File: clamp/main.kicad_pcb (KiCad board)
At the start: 2 copper layers, 80 parts, among them P1 CONN_01X12, P2 CONN_01X15, P3 CONN_01X03, P4 CONN_01X08, Q1 2N3904, U1 LM741, U12 LTZ1000, U13 LM741, U14 LM741, U2 LM741, U3 LM741, U4 LM741, U5 LM741, U6 LM741, U7 LM741

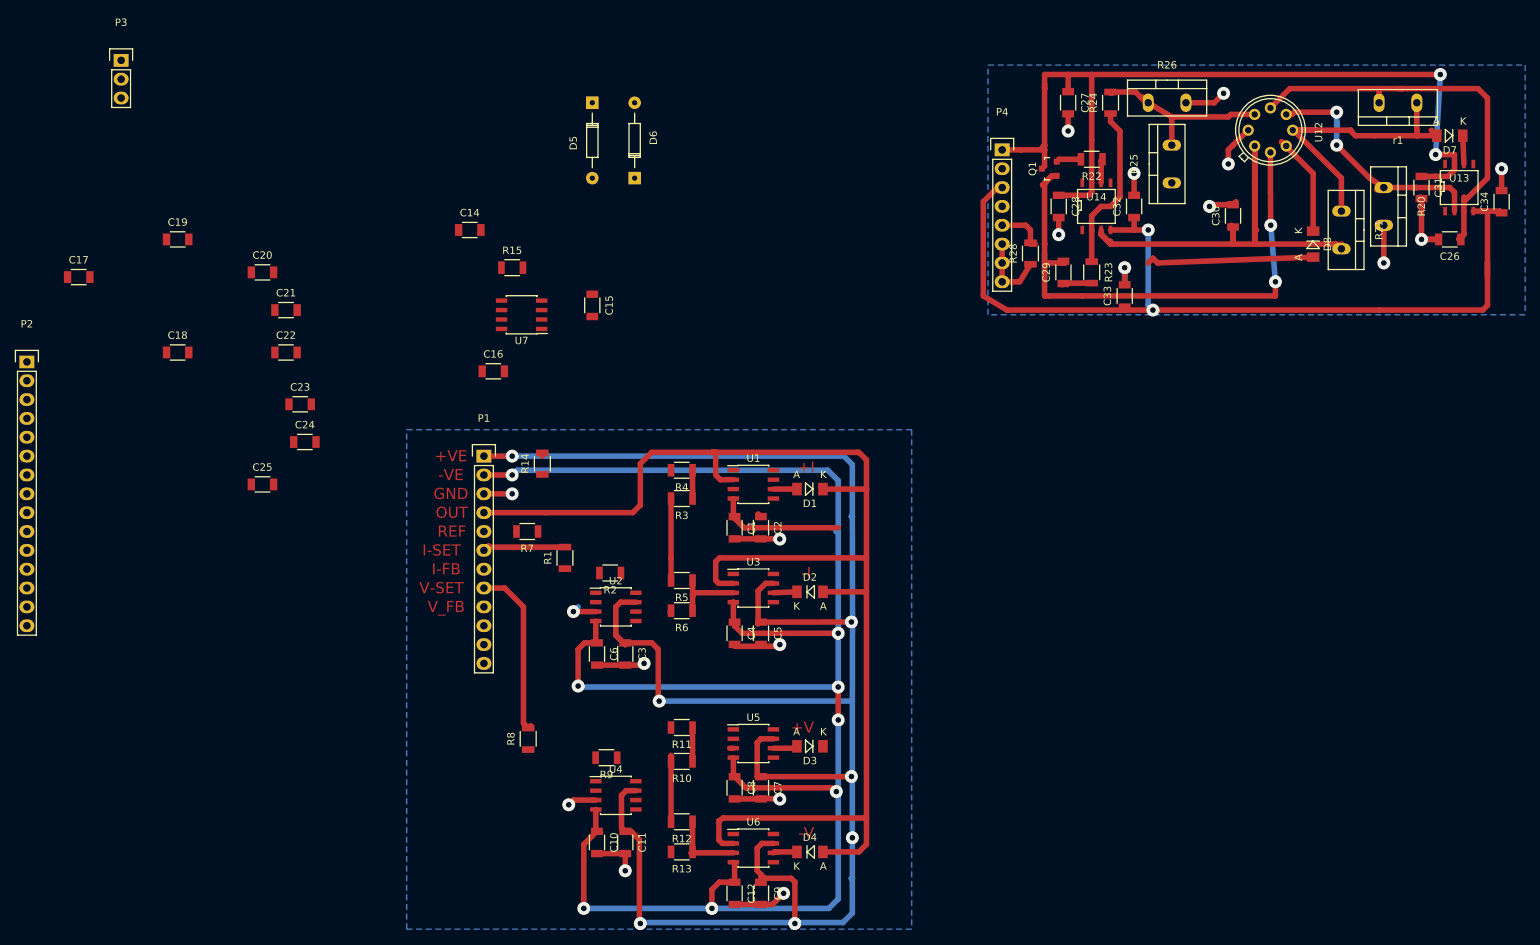
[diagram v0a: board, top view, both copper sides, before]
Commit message: update
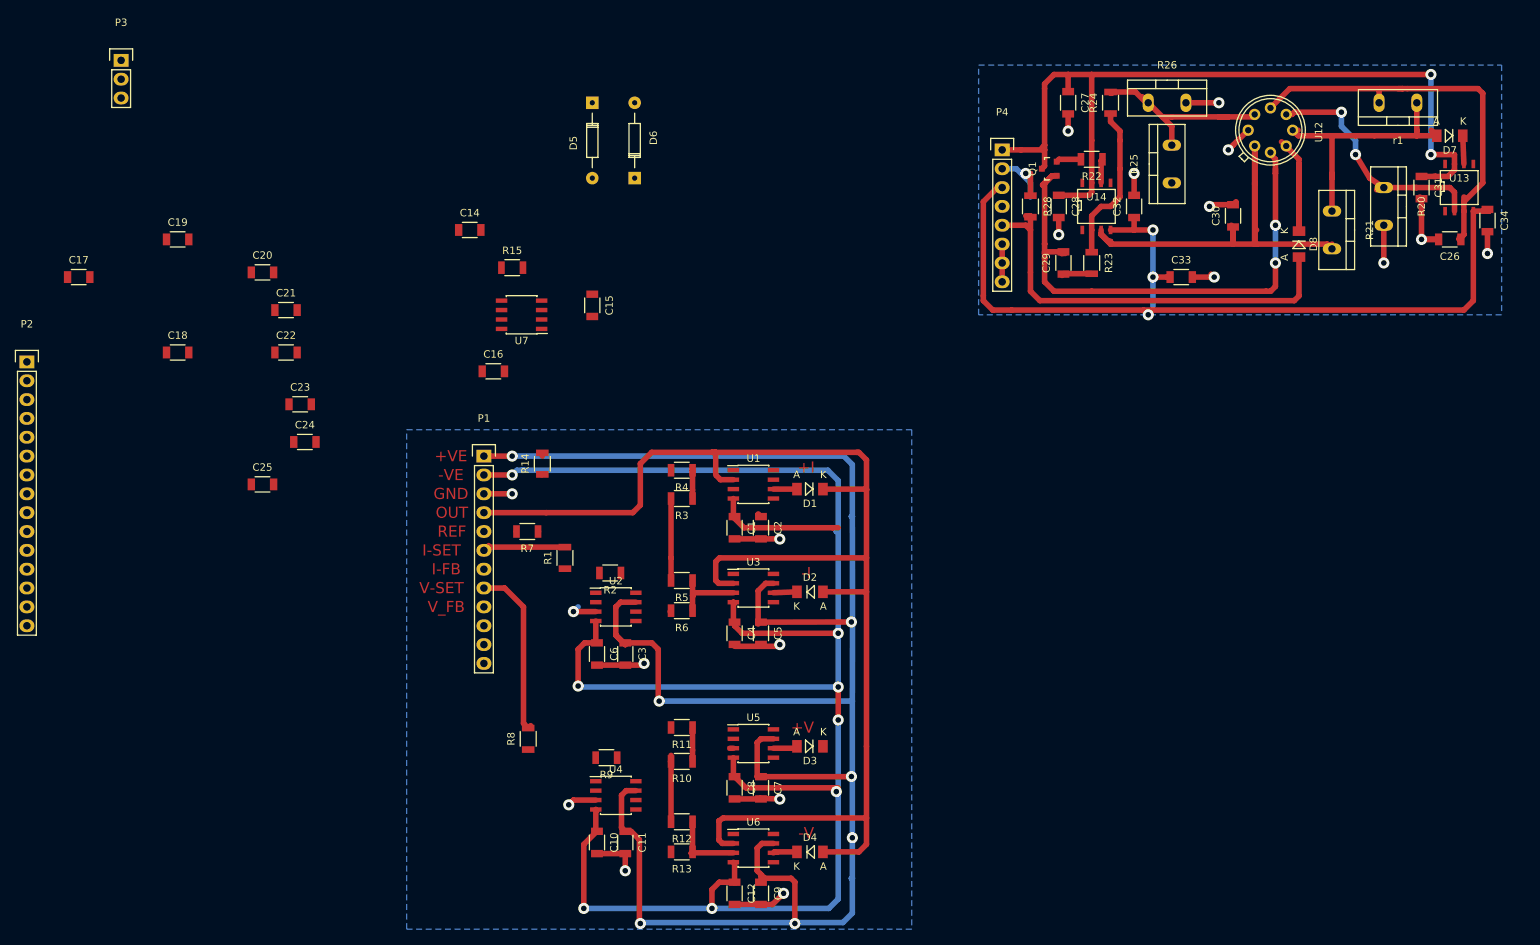
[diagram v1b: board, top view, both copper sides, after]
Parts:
- moved C33 8.03 mm to (212.1, 62.2), turned to 0 degrees
- moved R28 6.35 mm to (191.8, 52.7), turned to 270 degrees
- moved C34 3.18 mm to (253.4, 54.6), turned to 270 degrees
- moved D8 1.91 mm to (228.0, 57.8)
- moved R21 1.27 mm to (232.4, 55.9)
- moved C29 1.27 mm to (196.2, 60.3)
- moved R23 1.27 mm to (200.0, 60.3)
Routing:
- net GND-H: track 29.5 -> 57.2 mm
- net Net-(D8-Pad1): track 14.9 -> 22.2 mm
- net REF: track 43.7 -> 37.5 mm
- net (no net): track 3.40 -> 0.23 mm
- net Net-(R24-Pad2): track 27.2 -> 29.3 mm
- net +VE: track 399.6 -> 397.5 mm
- net Net-(C29-Pad2): track 73.7 -> 72.2 mm
- net Net-(R23-Pad1): track 23.3 -> 22.0 mm
- net Net-(C30-Pad1): track 69.8 -> 68.5 mm
- net GND: track 101.0 -> 101.7 mm, vias 18 -> 19
- net Net-(C26-Pad1): track 55.2 -> 54.7 mm
- net Net-(R20-Pad1): track 34.6 -> 34.0 mm
- net -VE: track 373.9 -> 373.4 mm, vias 10 -> 11
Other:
- net class Default: via_dia 1.75 -> 1.5

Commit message: update
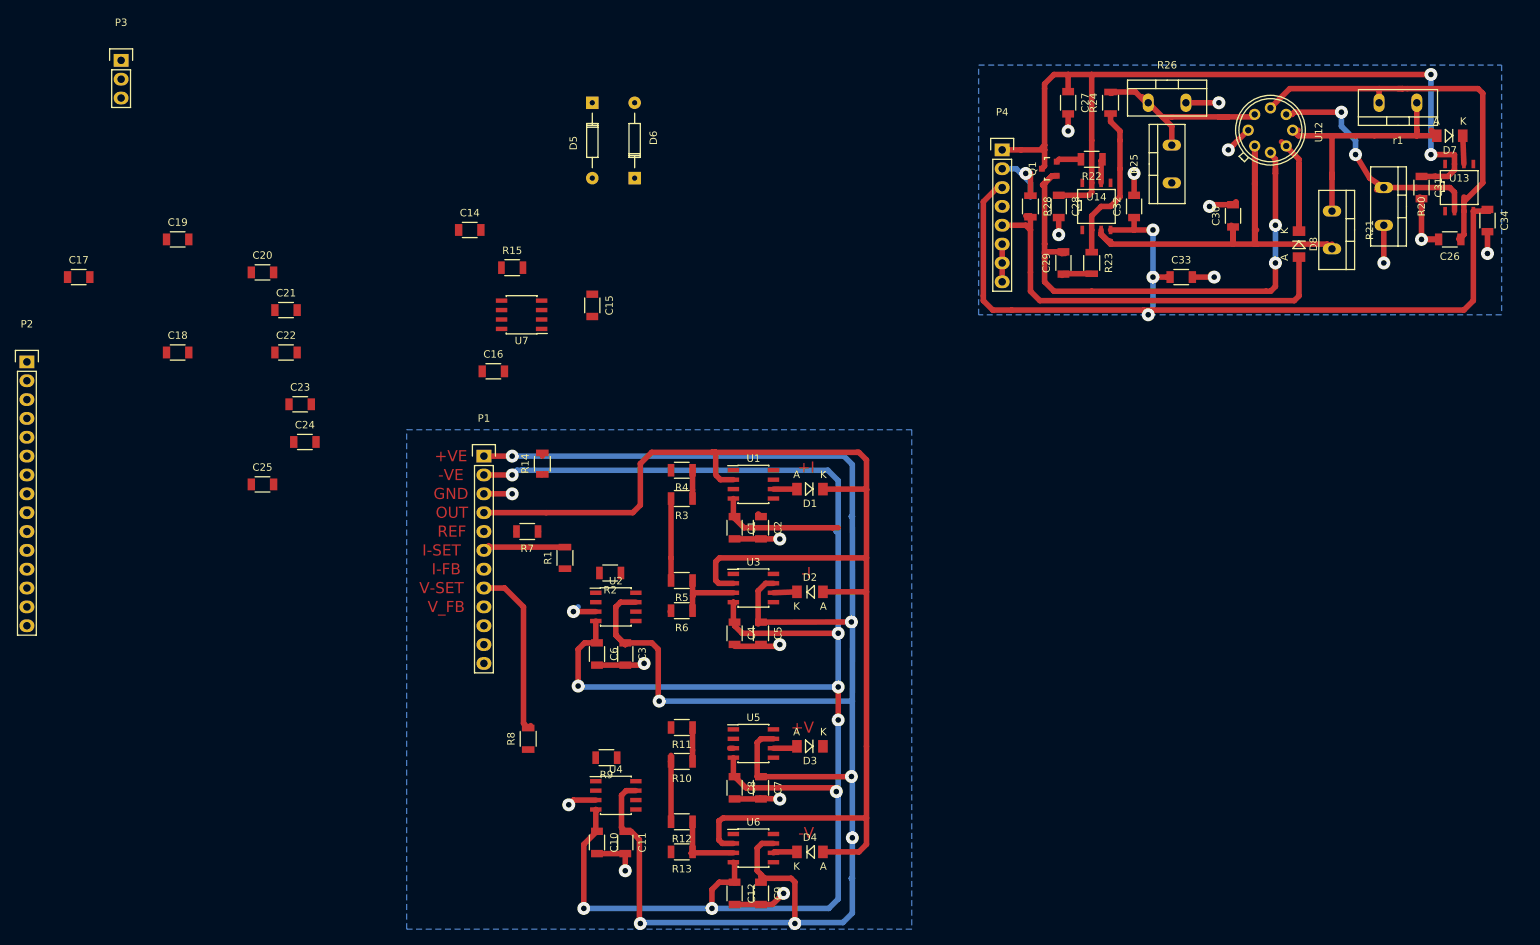
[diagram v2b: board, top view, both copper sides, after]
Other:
- net class Default: via_dia 1.5 -> 1.75

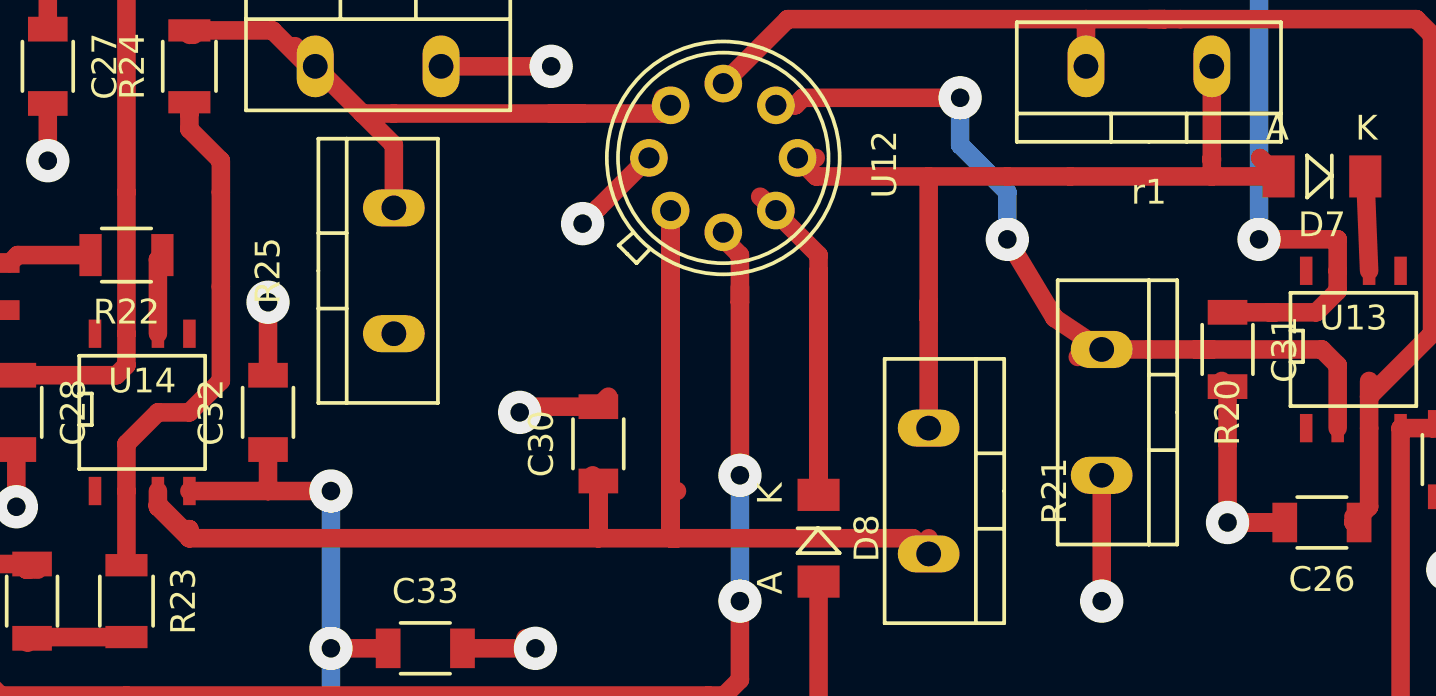
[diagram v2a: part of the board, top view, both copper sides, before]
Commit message: update
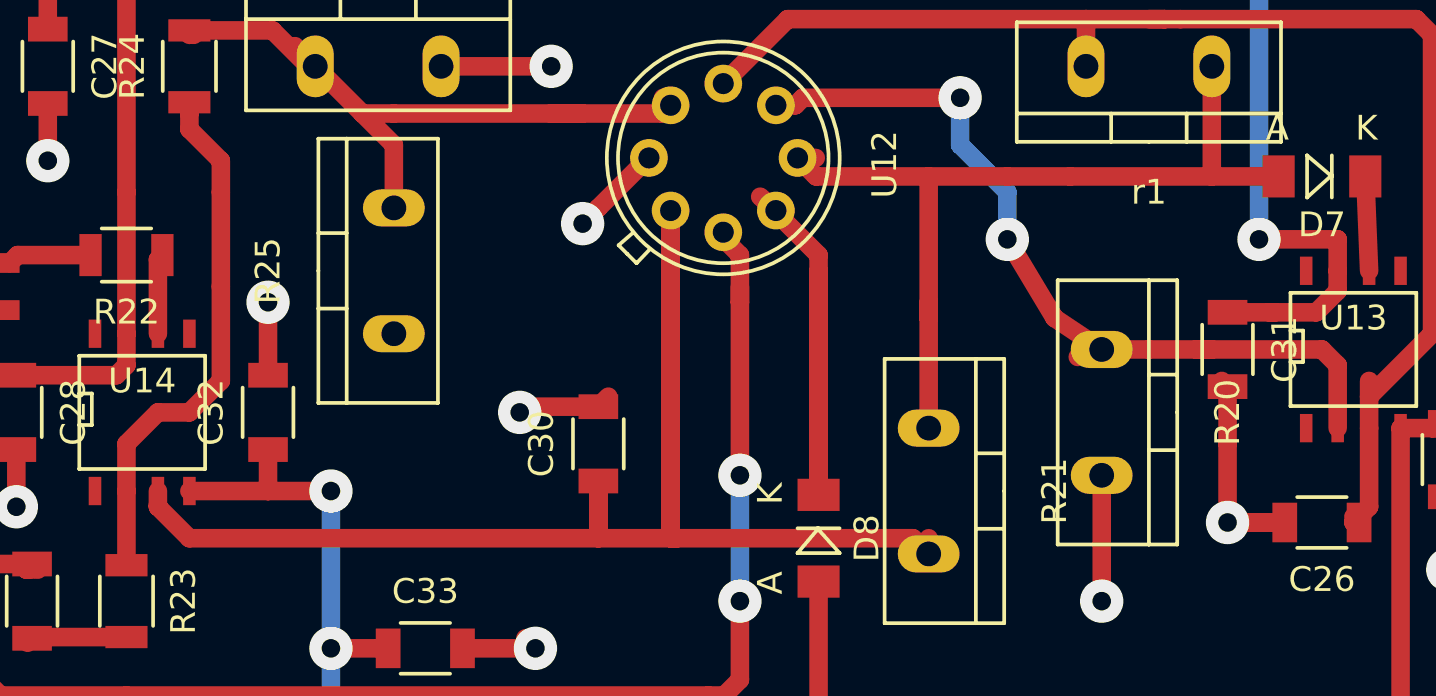
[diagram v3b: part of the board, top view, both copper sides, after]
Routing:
- net Net-(C30-Pad1): track 68.5 -> 65.9 mm
- net REF: track 37.5 -> 36.5 mm
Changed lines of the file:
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@@
     (thickness 1.6)
     (drawings 13)
-    (tracks 518)
+    (tracks 510)
     (zones 0)
     (modules 80)
@@
     (effects (font (size 1.5 1.5) (thickness 0.3)))
   )
-  (segment (start 243.84 42.4325) (end 243.84 42.545) (width 0.75) (layer F.Cu) (net 0))
-  (segment (start 243.84 42.545) (end 243.84 42.4325) (width 0.75) (layer F.Cu) (net 0))
   (segment (start 194.945 34.925) (end 193.675 36.195) (width 0.75) (layer F.Cu) (net 1))
   (segment (start 193.675 36.195) (end 193.675 36.83) (width 0.75) (layer F.Cu) (net 1))
@@
   (segment (start 149.352 85.852) (end 149.352 88.9) (width 0.75) (layer F.Cu) (net 5))
   (segment (start 149.479 89.027) (end 149.987 89.535) (width 0.75) (layer F.Cu) (net 5))
+  (segment (start 243.84 38.735) (end 243.84 43.18) (width 0.75) (layer F.Cu) (net 6))
   (segment (start 232.41 48.895) (end 232.41 43.18) (width 0.75) (layer F.Cu) (net 6))
   (segment (start 235.585 43.18) (end 232.41 43.18) (width 0.75) (layer F.Cu) (net 6))
@@
   (segment (start 232.41 48.26) (end 232.41 48.895) (width 0.75) (layer F.Cu) (net 6))
   (segment (start 232.41 48.895) (end 232.41 53.34) (width 0.75) (layer F.Cu) (net 6))
-  (segment (start 243.84 38.735) (end 243.84 43.18) (width 0.75) (layer F.Cu) (net 6))
   (segment (start 246.53494 43.18) (end 243.84 43.18) (width 0.75) (layer F.Cu) (net 6))
-  (segment (start 245.78744 42.4325) (end 246.53494 43.18) (width 0.75) (layer F.Cu) (net 6))
   (segment (start 227.1175 42.4325) (end 227.2175 42.4325) (width 0.75) (layer F.Cu) (net 6))
   (segment (start 227.1175 42.4325) (end 227.8525 42.4325) (width 0.75) (layer F.Cu) (net 6))
@@
   (segment (start 222.25 57.785) (end 219.075 57.785) (width 0.75) (layer F.Cu) (net 36))
   (segment (start 219.075 57.785) (end 202.565 57.785) (width 0.75) (layer F.Cu) (net 36))
-  (segment (start 202.565 57.785) (end 202.565 57.419998) (width 0.75) (layer F.Cu) (net 36))
   (segment (start 221.9925 55.88) (end 221.9925 57.419998) (width 0.75) (layer F.Cu) (net 36))
-  (segment (start 202.565 57.419998) (end 202.295002 57.419998) (width 0.75) (layer F.Cu) (net 36))
-  (segment (start 202.295002 57.419998) (end 201.295 56.419996) (width 0.75) (layer F.Cu) (net 36))
   (segment (start 201.295 56.419996) (end 201.295 56.515) (width 0.75) (layer F.Cu) (net 36))
   (segment (start 219.075 55.475) (end 219.075 57.419998) (width 0.75) (layer F.Cu) (net 36) (status 10))
@@
   (segment (start 218.845 55.475) (end 219.075 55.475) (width 0.75) (layer F.Cu) (net 36) (status 30))
   (segment (start 221.9925 49.53) (end 221.9925 55.88) (width 0.75) (layer F.Cu) (net 36))
-  (segment (start 221.9925 55.88) (end 222.25 55.88) (width 0.75) (layer F.Cu) (net 36))
   (segment (start 221.9925 44.5575) (end 221.9925 49.53) (width 0.75) (layer F.Cu) (net 36))
   (segment (start 221.9925 49.53) (end 221.9925 49.7875) (width 0.75) (layer F.Cu) (net 36))
-  (segment (start 218.845 55.245) (end 219.075 55.475) (width 0.75) (layer F.Cu) (net 36) (status 30))
   (segment (start 232.6675 58.6775) (end 232.41 58.42) (width 0.75) (layer F.Cu) (net 36) (status 30))
   (segment (start 232.6675 58.6775) (end 232.41 58.42) (width 0.75) (layer B.Cu) (net 36) (status 30))
